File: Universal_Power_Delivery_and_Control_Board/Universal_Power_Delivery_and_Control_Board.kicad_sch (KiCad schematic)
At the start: 19 parts, among them U17 SN74LVC1G17DCKR, U19 TF-0803-0, U20 TCA9555PWR

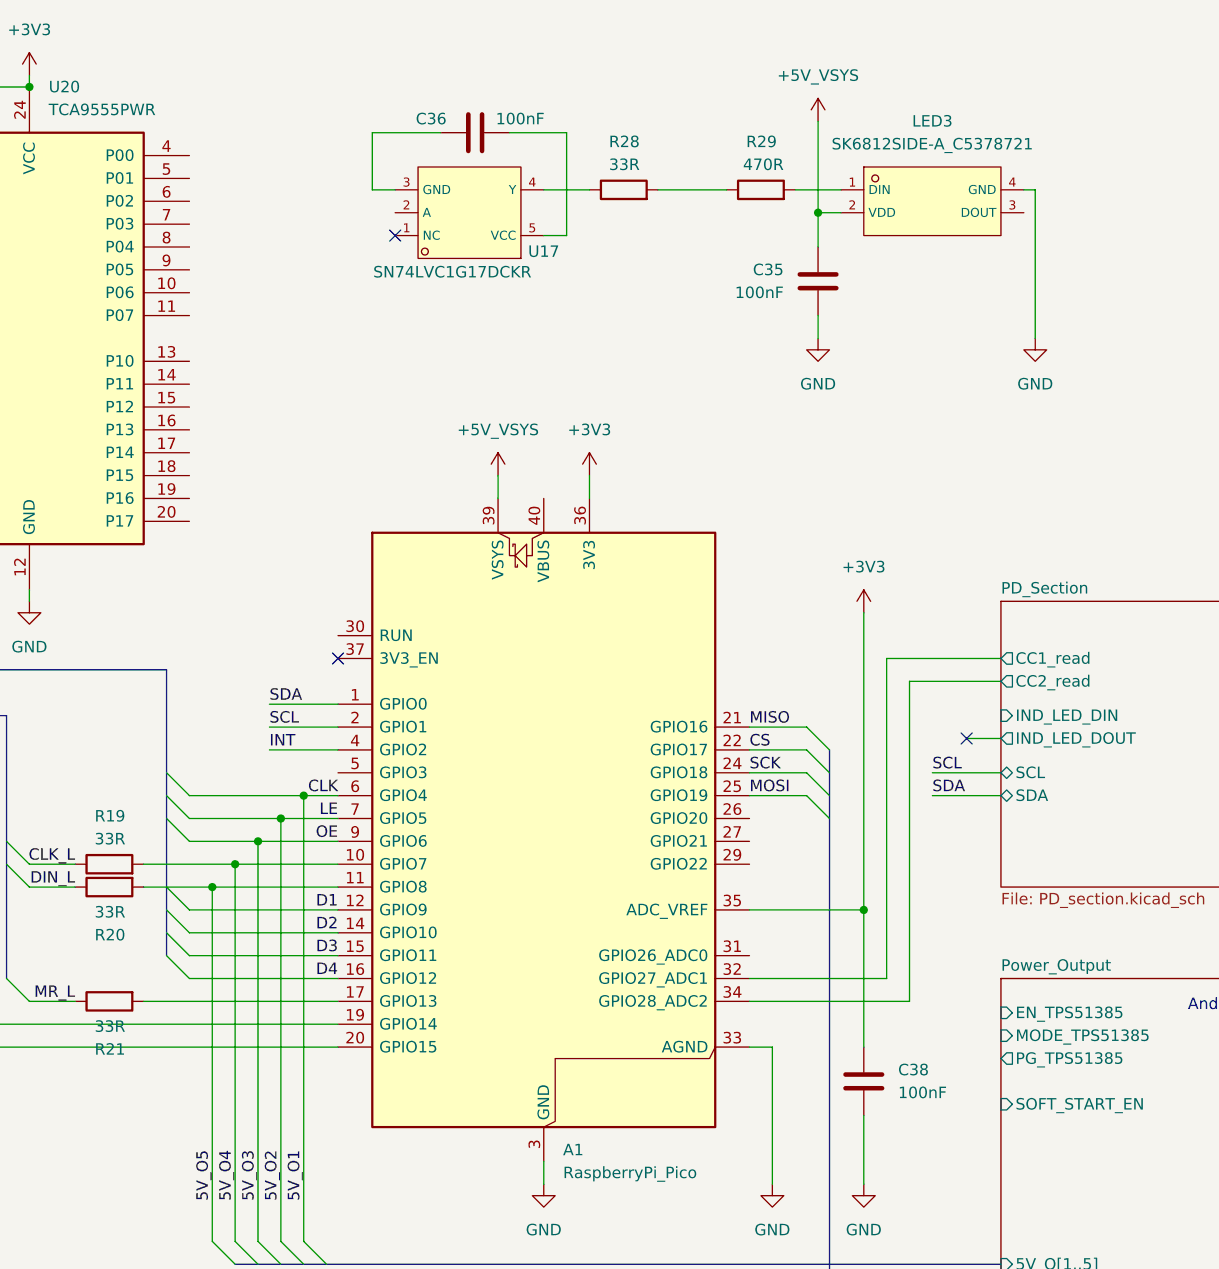
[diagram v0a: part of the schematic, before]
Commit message: Added some misc stuff layout almost finished.
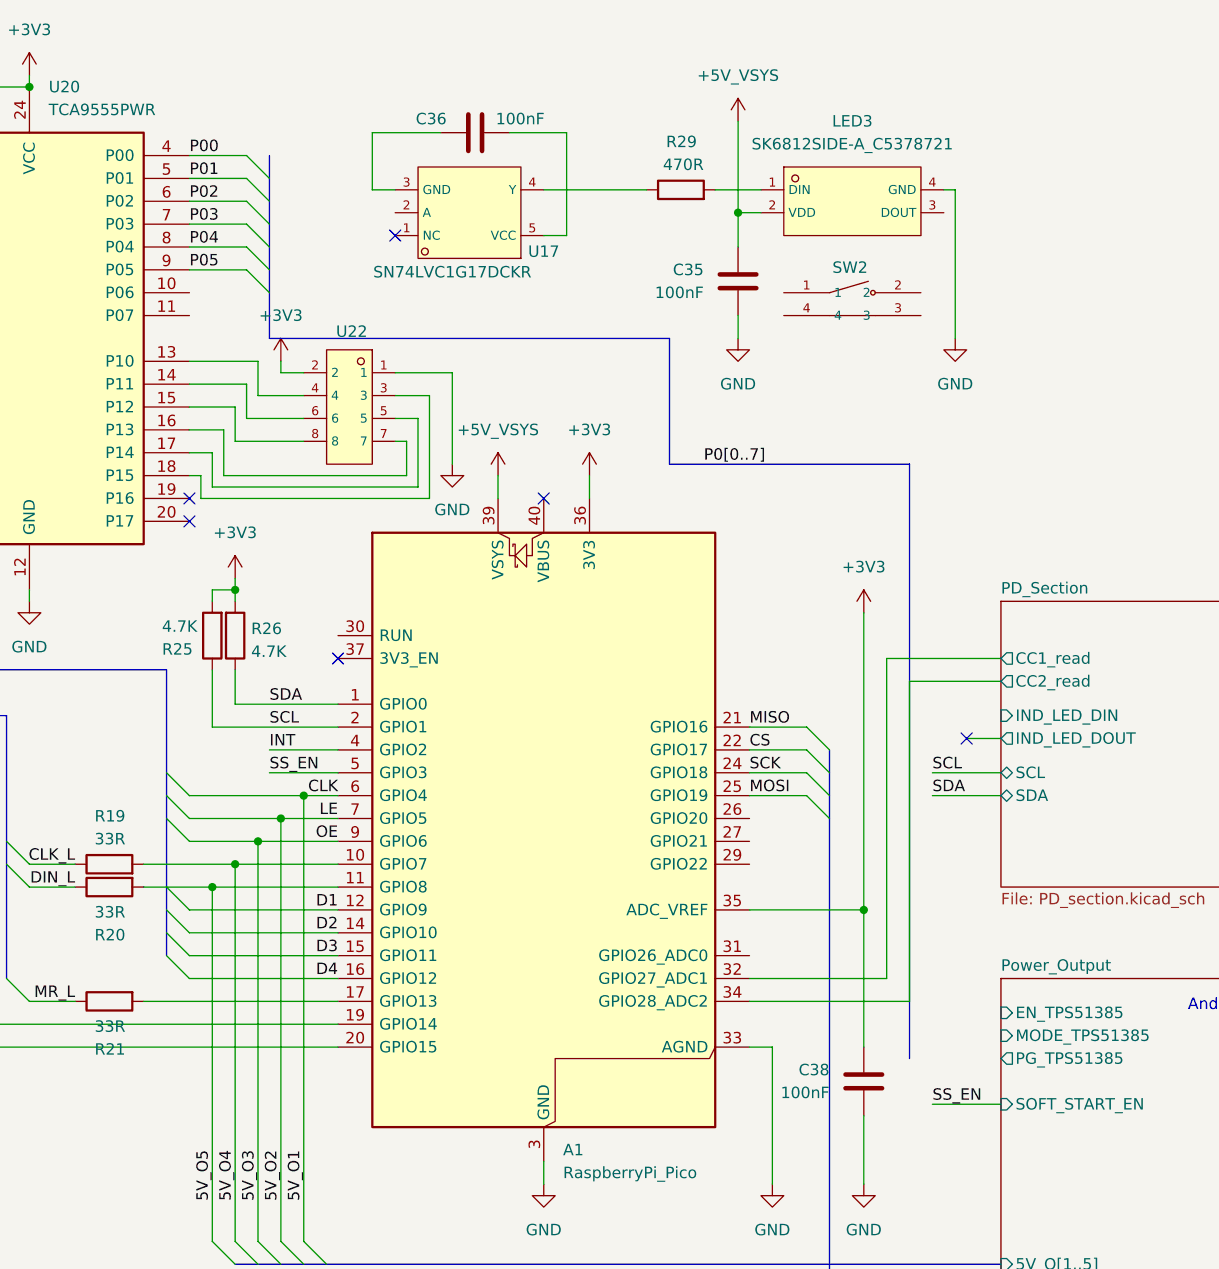
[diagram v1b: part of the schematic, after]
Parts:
- removed R28: 33R, Resistor_SMD:R_0402_1005Metric_Pad0.72x0.64mm_HandSolder, symbol Device:R
- added R25, R26: 4.7K, Resistor_SMD:R_0402_1005Metric_Pad0.72x0.64mm_HandSolder, symbol Device:R
- added SW2: TS1102-TD35HBM, lcsc_footprints:C36936640_SW-SMD_TS1102-TD35HBM, symbol lcsc_imported:TS1102-TD35HBM
- added U22: HC-PM254-8.5H-2X4PW-02A, lcsc_footprints:C42163146_HDR-TH_8P-P2_54-H-F-R2-C4-S2_54-W8_5, symbol lcsc_imported:HC-PM254-8_5H-2X4PW-02A
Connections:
- net +3V3: now also R25.2, R26.2, U22.2
- net GND: now also U22.1
- net SCL: now also R25.1
- net SDA: now also R26.1
- net at U20.13 (P10): now also U22.4
- net at U20.14 (P11): now also U22.6
- net at U20.15 (P12): now also U22.8
- net at U20.16 (P13): now also U22.7
- net at U20.17 (P14): now also U22.5
- net at U20.18 (P15): now also U22.3
- net P00: now reaches U20.4 (P00)
- net P01: now reaches U20.5 (P01)
- net P02: now reaches U20.6 (P02)
- net P03: now reaches U20.7 (P03)
- net P04: now reaches U20.8 (P04)
- net P05: now reaches U20.9 (P05)
- net SS_EN: now reaches A1.5 (GPIO3)
- net at R29.1: now also U17.4 (Y)
- no-connect marks 6 -> 9
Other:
- moved on the sheet: C35, LED3, R29
